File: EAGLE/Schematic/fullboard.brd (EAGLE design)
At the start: 89.5 x 77.1 mm, 91 parts, among them CN1 B4B-ZR, CN2 B4B-ZR, CN3 B4B-ZR, IC1 IFX007T, IC2 IFX007T, IC3 IFX007T, IC4 IFX007T, IC5 FT232RL-REEL, IC6 LDL1117S33R, IC7 AZ1117IH, J1 10118193-0001LF, Q1 8MHz ±10ppm Crystal 18pF 80 O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, Q2 AOD4189, SW1 TR1-SPST, U1 ATXMEGA128A3U-AU

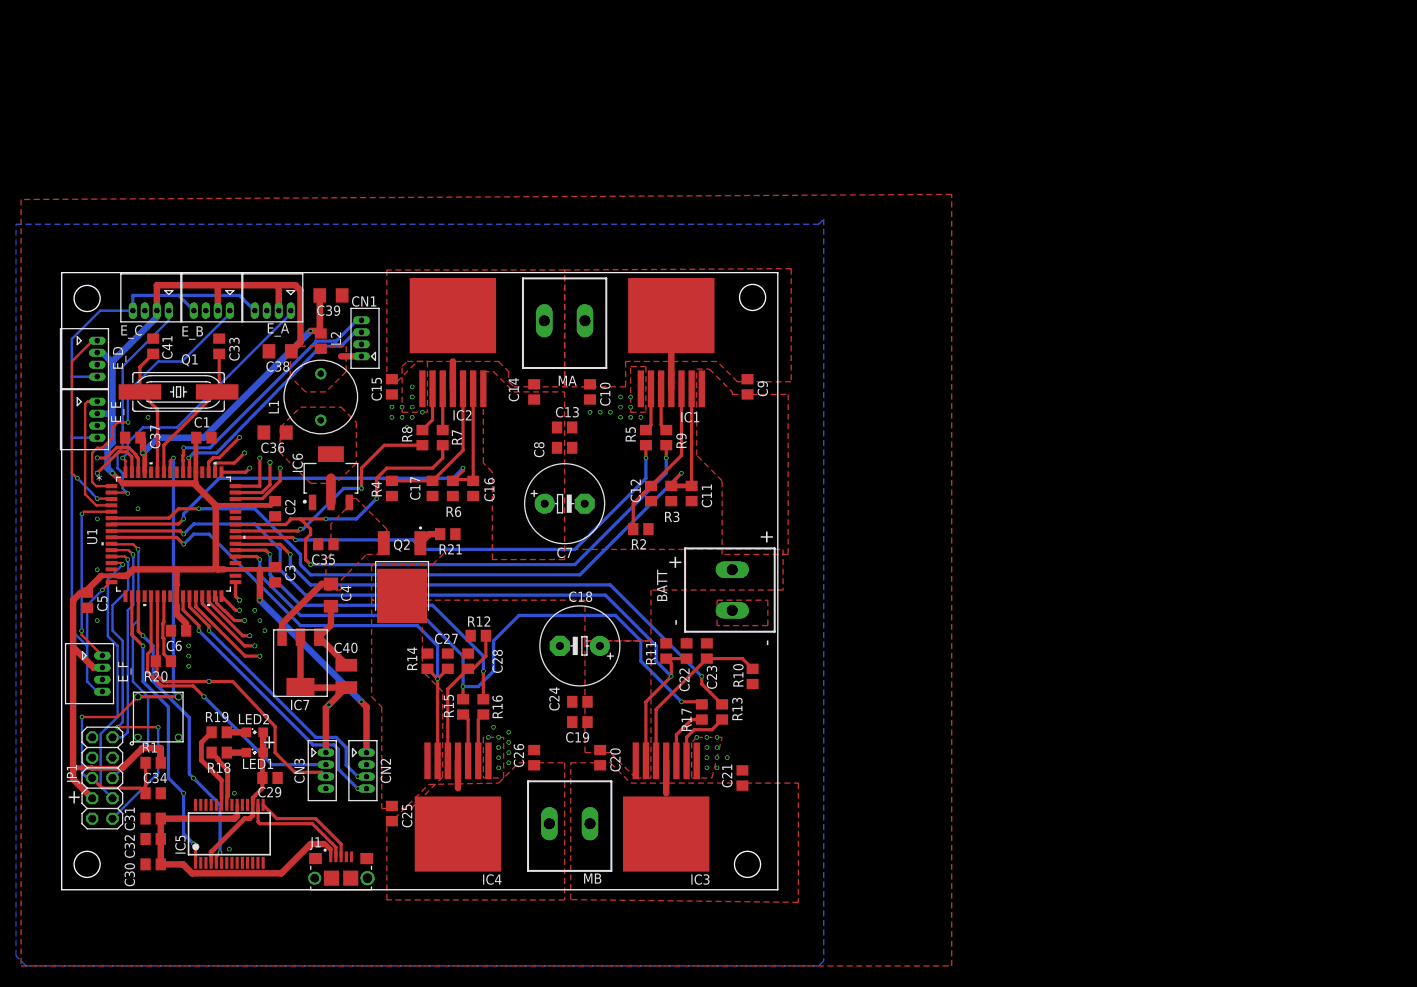
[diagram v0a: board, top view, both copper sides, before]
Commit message: V1.0
Final version board design
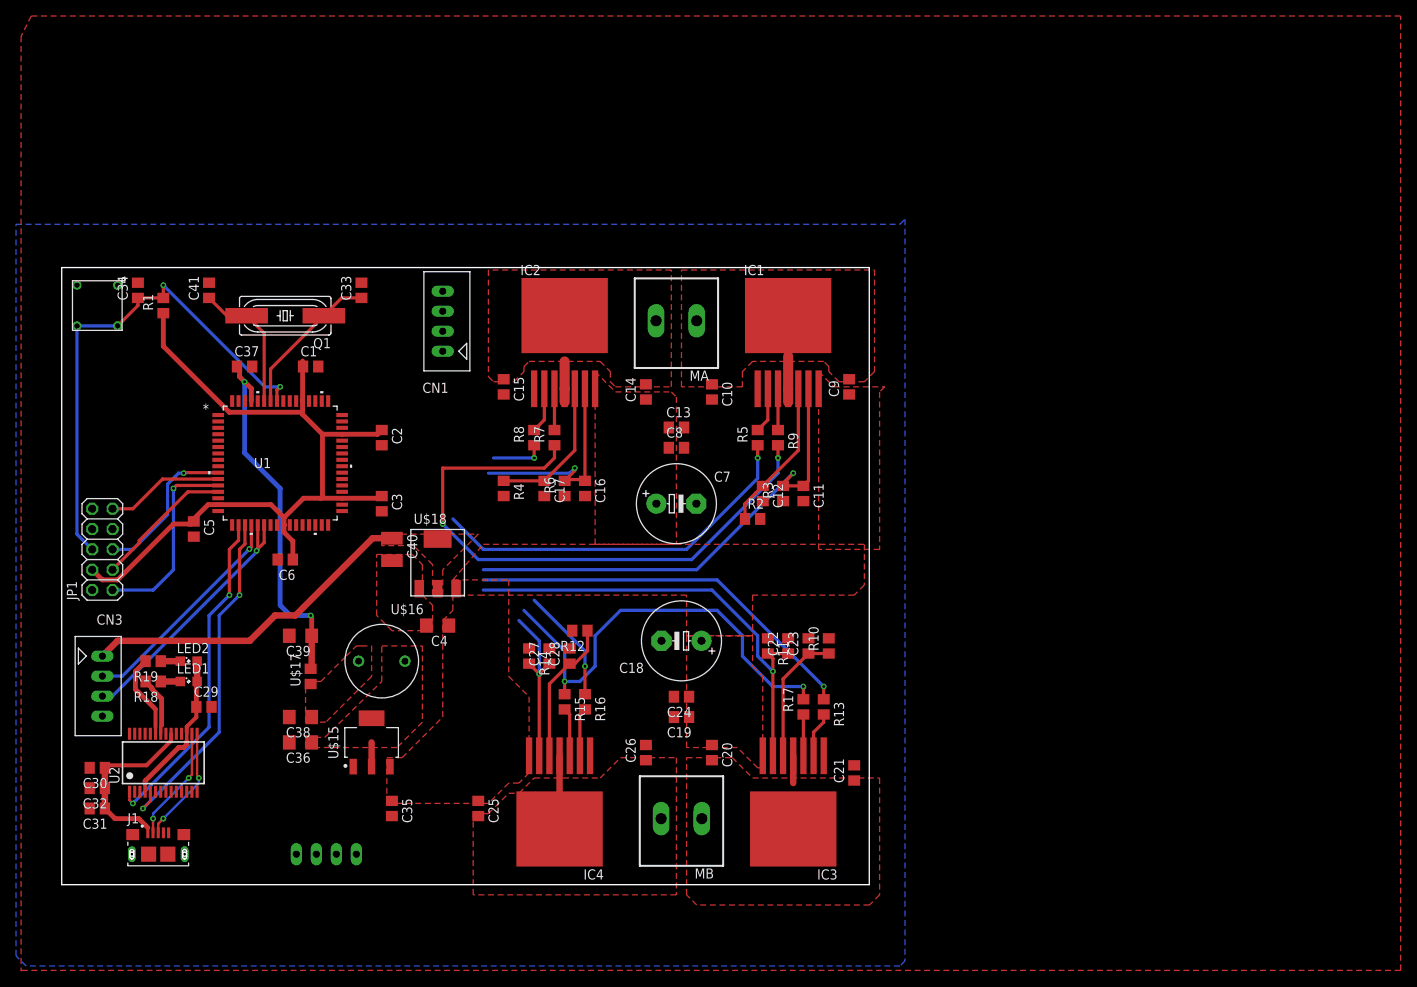
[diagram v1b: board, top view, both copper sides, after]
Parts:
- removed BATT: (no value), ME507:2POL508
- removed E_A, E_B, E_C, E_D, E_E, E_F: S4B-ZR, jst:S4B-ZR
- removed IC5: FT232RL-REEL, FT232RL-REEL:SOP65P780X200-28N
- removed IC6: LDL1117S33R, SumBot:SOT230P700X190-4N
- removed IC7: AZ1117IH, SumBot:SOT223
- removed L1: RLB0914-100KL, SumBot:INDRD580W65D870H1300B
- removed L2: BLM21PG221SN1D, blm21:C0805
- removed Q2: AOD4189, AOD4189:AOD480
- removed R20: 47Ω, rcl:R0805
- removed R21: 10kΩ, rcl:R0805
- added U$15: LDL1117S33R, SumBot:SOT230P700X190-4N
- added U$16: RLB0914-100KL, SumBot:INDRD580W65D870H1300B
- added U$17: BLM21PG221SN1D, blm21:C0805
- added U$18: AZ1117IH, SumBot:SOT223
- added U2: FT232RL-REEL, FT232RL-REEL:SOP65P780X200-28N
- CN1, CN2, CN3: value B4B-ZR -> B4B-XH-A; device jst:B4B-ZR -> jst:B4B-XH-A
- moved C34 62.9 mm to (9.53, 74.9), turned to 90 degrees
- moved R1 57.2 mm to (12.7, 73.0), turned to 90 degrees
- moved SW1 52.0 mm to (4.45, 73.0), turned to 90 degrees
- moved C38 45.8 mm to (29.8, 21.6)
- moved C39 42.7 mm to (29.8, 31.8), turned to 180 degrees
- moved C36 38.9 mm to (29.8, 18.4)
- moved C35 34.0 mm to (41.3, 10.2), turned to 270 degrees
- moved CN3 30.4 mm to (5.08, 29.2)
- moved JP1 28.6 mm to (5.08, 42.5)
- moved J1 23.1 mm to (12.1, 4.45)
- moved C33 19.1 mm to (37.5, 74.9)
- moved C40 16.9 mm to (41.3, 42.5), turned to 270 degrees
- moved C37 16.6 mm to (22.9, 65.4), turned to 0 degrees
- moved Q1 16.4 mm to (27.9, 71.8)
- moved C2 16.0 mm to (40.0, 56.5)
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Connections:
- removed net EDGE_CTRL: E_A.4, E_B.4, E_C.4, E_D.4, E_E.4, E_F.4, U1.16
- removed net N$14: R20.1, U1.23
- removed net N$36: C35.1, C4.1, IC6.3, IC7.3, Q2.3
- removed net N$37: Q2.1, R21.2
- removed net N$38: U1.46
- removed net N$39: U1.47
- removed net N$40: U1.48
- removed net N$41: U1.49
- removed net N$42: U1.50
- removed net N$43: U1.51
- removed net N$44: U1.33
- removed net N$45: U1.32
- removed net N$46: U1.31
- removed net N$47: U1.30
- removed net N$48: U1.29
- removed net N$49: U1.28
- removed net N$50: U1.62
- removed net N$51: U1.63
- new net CS_A: C11.1, C16.1, IC1.6, IC2.6, R3.2, R6.2
- new net CS_B: C22.1, C27.1, IC3.6, IC4.6, R11.2, R14.2
- net +12V: now also C35.1, C4.1, U$15.3, U$18.3; no longer BATT.2, Q2.2
- net +3V3: now also U$16.1, U$17.1; no longer E_A.2, E_B.2, E_C.2, E_D.2, E_E.2, E_F.2, L1.1, L2.1
- net +5V: now also U$18.2, U$18.4; no longer IC7.2, IC7.4
- net AVCC: now also U$17.2; no longer L2.2
- net BCK_A: now also U1.27; no longer U1.41
- net BCK_B: now also U1.29; no longer U1.38
- net CSB_A: no longer C16.1, IC2.6, R6.2
- net CSB_B: no longer C27.1, IC4.6, R14.2
- net CSF_A: no longer C11.1, IC1.6, R3.2
- net CSF_B: no longer C22.1, IC3.6, R11.2
- net EA_A: now also U1.50; no longer U1.54
- net EA_B: now also U1.47; no longer U1.27
- net EB_A: now also U1.51; no longer U1.55
- net EB_B: now also U1.48; no longer U1.26
- net EDGE_A: now also U1.62; no longer E_A.1, U1.64
- net EDGE_B: now also U1.63; no longer E_B.1, U1.1
- net EDGE_C: now also U1.64; no longer E_C.1, U1.2
- net EDGE_D: now also U1.1; no longer E_D.1, U1.3
- net EDGE_E: now also U1.2; no longer E_E.1, U1.4
- net EDGE_F: now also U1.3; no longer E_F.1, U1.5
- net EN_A: now also U1.49; no longer U1.42
- net EN_B: now also U1.46; no longer U1.37
- net FWD_A: now also U1.26; no longer U1.40
- net FWD_B: now also U1.28; no longer U1.39
- net GND: now also U$15.1, U2.18, U2.21, U2.25, U2.26, U2.7; no longer BATT.1, E_A.3, E_B.3, E_C.3, E_D.3, E_E.3, E_F.3, IC5.18, IC5.21, IC5.25, IC5.26, IC5.7, IC6.1, R21.1
- net N$1: now also U$18.1; no longer IC7.1
- net N$18: now also U2.16; no longer IC5.16
- net N$19: now also U2.15; no longer IC5.15
- net N$21: now also U2.23; no longer IC5.23
- net N$22: now also U2.22; no longer IC5.22
- net N$24: now also U2.27; no longer IC5.27
- net N$25: now also U2.9; no longer IC5.9
- net N$26: now also U2.11; no longer IC5.11
- net N$27: now also U2.28; no longer IC5.28
- net N$28: now also U2.2; no longer IC5.2
- net N$29: now also U2.3; no longer IC5.3
- net N$30: now also U2.13; no longer IC5.13
- net N$31: now also U2.14; no longer IC5.14
- net N$32: now also U2.12; no longer IC5.12
- net N$33: now also U2.6; no longer IC5.6
- net N$34: now also U2.10; no longer IC5.10
- net N$35: now also U2.19; no longer IC5.19
- net N$8: now also U$15.2, U$15.4, U$16.2; no longer IC6.2, IC6.4, L1.2
- net RX_FT232: now also U2.1; no longer IC5.1
- net TX/RX_MSE: now also U1.21; no longer R20.2
- net TX_FT232: now also U2.5; no longer IC5.5
- net USB_PWR: now also U2.20; no longer IC5.20
- net VCCIO: now also U2.17, U2.4; no longer IC5.17, IC5.4
- net XCK_MSE: now also U1.20; no longer U1.21
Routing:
- net +3V3: track 212.1 -> 99.9 mm, vias 3 -> 0
- net CSF_B: track 98.1 -> 0.00 mm, vias 2 -> 0
- net CSF_A: track 98.0 -> 0.00 mm, vias 2 -> 0
- net EDGE_CTRL: track 91.4 -> 0.00 mm, vias 1 -> 0
- net CS_A: track 0.00 -> 88.8 mm, vias 0 -> 2
- net CS_B: track 0.00 -> 79.0 mm, vias 0 -> 2
- net CSB_B: track 65.4 -> 0.00 mm, vias 2 -> 0
- net CSB_A: track 63.5 -> 0.00 mm, vias 2 -> 0
- net EB_B: track 35.7 -> 0.00 mm, vias 2 -> 0
- net EDGE_B: track 34.1 -> 0.00 mm, vias 1 -> 0
- net EA_B: track 33.9 -> 0.00 mm, vias 2 -> 0
- net EB_A: track 32.0 -> 0.00 mm, vias 1 -> 0
- net EDGE_A: track 31.5 -> 0.00 mm, vias 1 -> 0
- net EA_A: track 30.0 -> 0.00 mm, vias 1 -> 0
- net BCK_B: track 43.4 -> 14.4 mm, vias 2 -> 1
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- added copper zone on layer 1, net +5V
- added copper zone on layer 1, net N$1
- removed copper zone on layer 1, net N$36
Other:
- board size 89.5 x 77.1 mm -> 100.9 x 77.1 mm
- board text removed: "+"
- board text removed: "+3.3V"
- board text removed: "+5V"
- board text removed: "-"
- board text removed: "0"
- board text removed: "2"
- board text removed: "3"
- board text removed: "7"
- board text removed: "AVCC"
- board text removed: "CLK"
- board text removed: "California Polytechnic State University of San Luis Obispo ME 507 - Mechanical Control System Design Fall 2019 - SumoBot v1.0 Ryan Forsberg & Philippe Habets"
- board text removed: "FT232"
- board text removed: "MSE"
- board text removed: "PA0"
- board text removed: "PA1"
- board text removed: "PD"
- board text removed: "PF"
- board text removed: "RX"
- board text removed: "TX"
- board text removed: "TX/RX"
